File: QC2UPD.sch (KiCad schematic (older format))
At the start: 16 parts

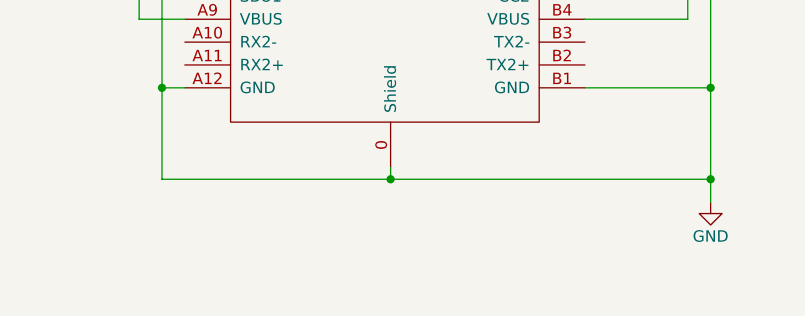
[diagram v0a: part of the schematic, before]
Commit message: Add USB-PD comment
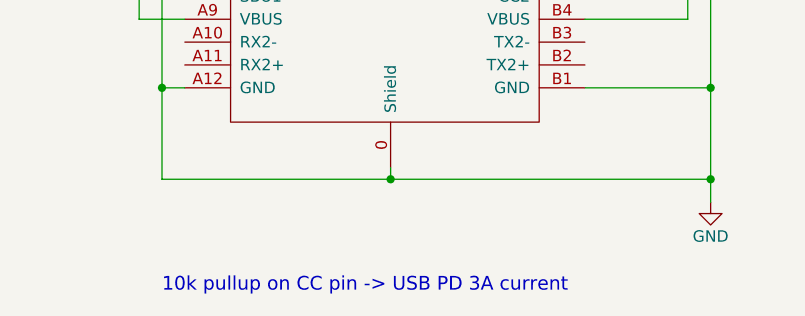
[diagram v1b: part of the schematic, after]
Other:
- note added: "10k pullup on CC pin -> USB PD 3A current"
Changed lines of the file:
@@
 Wire Wire Line
 	1700 1400 1700 1000
+Text Notes 8000 4400 0    60   ~ 0
+10k pullup on CC pin -> USB PD 3A current
 $EndSCHEMATC
